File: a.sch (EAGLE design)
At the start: 22 parts, among them SW1 TS6601-9,5, SW2 TS6601-9,5, U1 ESP32-WROVER-IE, X1 PLS-09, X2 PLS-07, X3 PLS2-6, X4 PLD-06

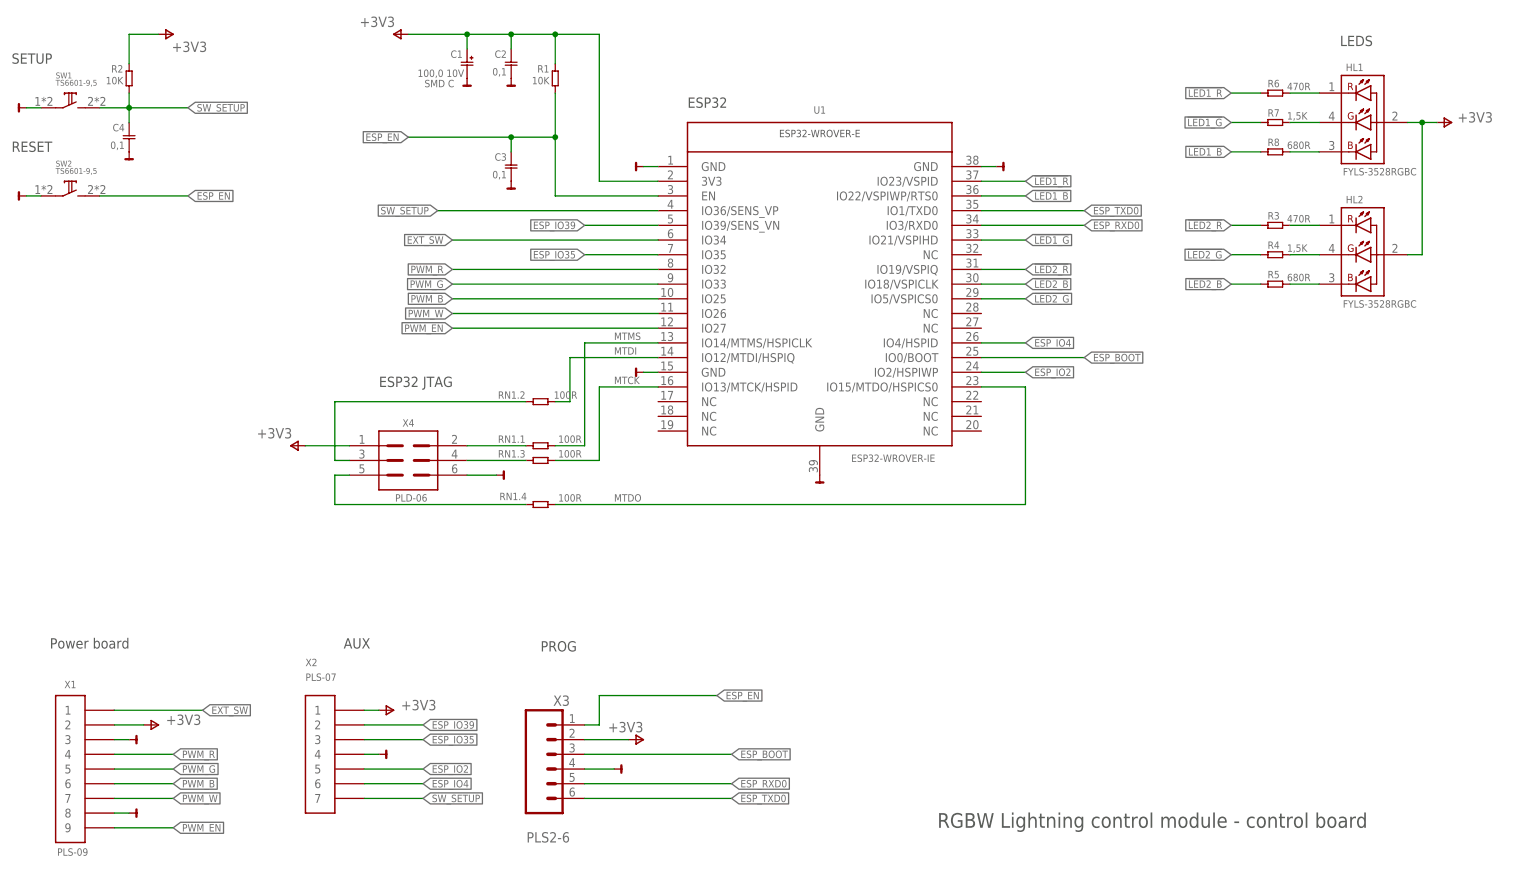
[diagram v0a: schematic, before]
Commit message: more import
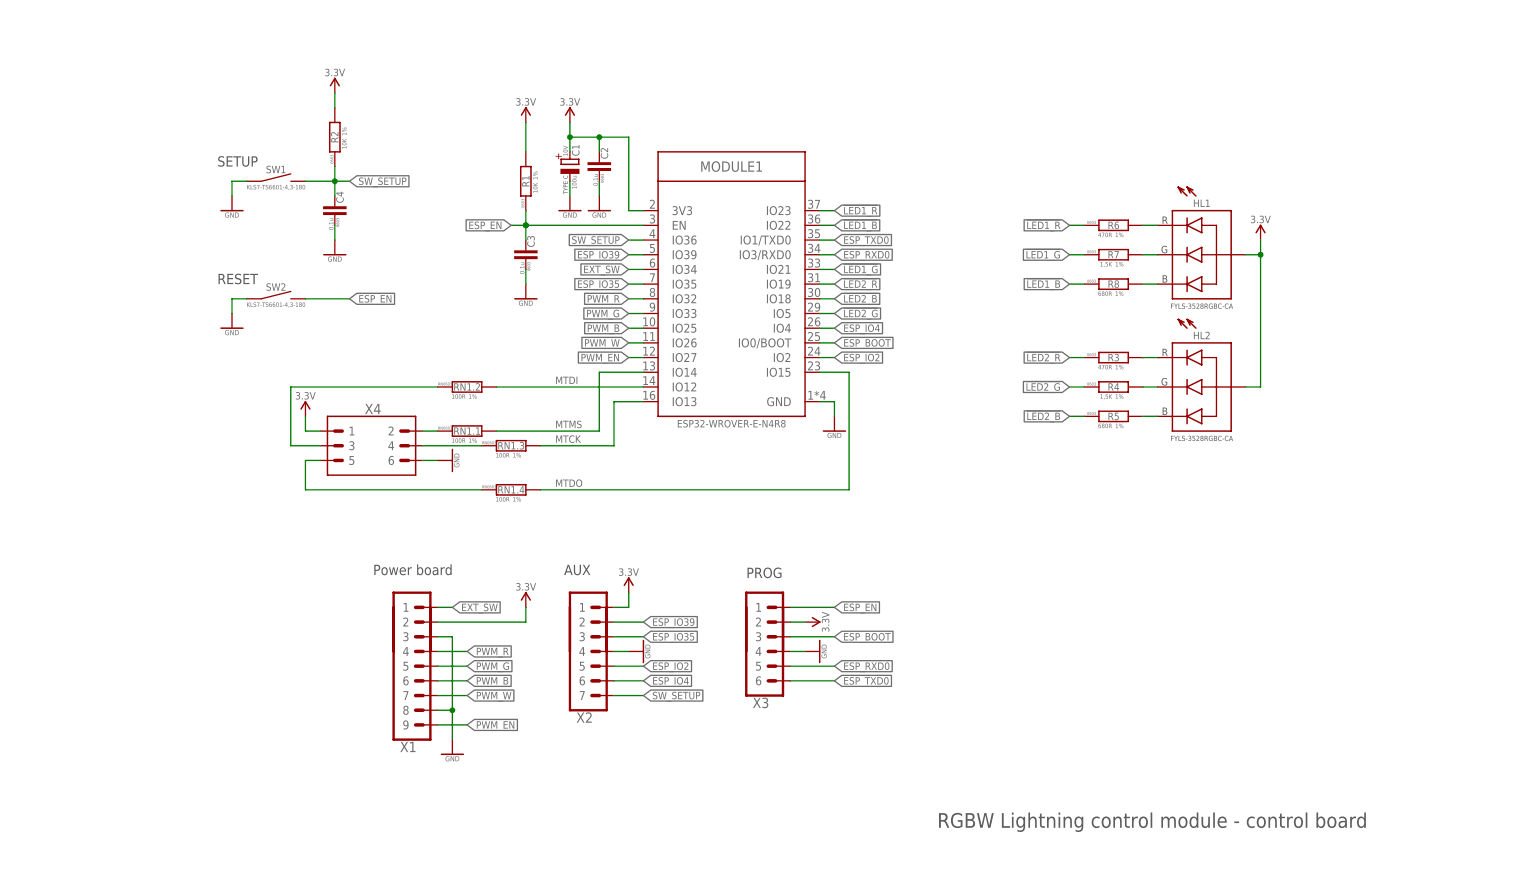
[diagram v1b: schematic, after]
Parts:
- removed U1: ESP32-WROVER-IE, pds019_lit:ESP32-WROVER-(I)E
- added MODULE1: ESP32-WROVER-(I)E, ali_modules:ESP32-WROVER-(I)E
- C1: value 100,0 10V -> 100u; device pds019_lit:CTANT_C -> rc:CPOL-TANT-TYPE-C; PKG SMD C -> (none); VOLTAGE (none) -> 10V
- C2, C3, C4: value 0,1 -> 0.1u; device pds019_lit:C0603 -> rc:C-0603; PKG 0603 -> (none); TOL -20/+80% -> (none); TYPE Y5V -> (none)
- HL1, HL2: value FYLS-3528RGBC -> LED_RGB-3528; device pds019_lit:FYLS-3528RGBC -> rc:LED_RGB-3528
- R1, R2, R3, R4, R5, R6, R7, R8: device pds019_lit:R0603 -> rc:R-1%-0603; PKG 0603 -> (none); TOL 5% -> (none)
- RN1: device pds019_lit:RN4X1_EXP-YC164 -> rc:RN-1%-0603
- SW1, SW2: device pds019_lit:SW_BUTTON -> mechanical:TACT_SWITCH-6X6-PTH
- X1: value PLS-09 -> PINHEAD_1X09-2.54-TH-MALE; device pds019_lit:PLS-09 -> pinhead:PINHEAD_1X09-2.54-TH-MALE
- X2: value PLS-07 -> PINHEAD_1X07-2.54; device pds019_lit:PLS-07 -> pinhead:PINHEAD_1X07-2.54
- X3: value PLS2-6 -> PINHEAD_1X06-2-MALE; device pds019_lit:PLS2-6 -> pinhead:PINHEAD_1X06-2-MALE
- X4: value PLD-06 -> PINHEAD_2X03-PTH-2.54; device pds019:PLD-06 -> pinhead:PINHEAD_2X03-PTH-2.54
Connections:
- removed net +3V3: C1.+, C2.2, HL1.A, HL2.A, R1.P$2, R2.P$2, U1.3V3, X1.2, X2.1, X3.2, X4.1
- new net VDD_3V3: C1.+, C2.2, HL1.A, HL2.A, MODULE1.3V3, R1.2, R2.2, X1.2, X2.1, X3.2, X4.1
- net !LED1_B: now also MODULE1.IO22, R8.1; no longer R8.P$1, U1.IO22/VSPIWP/RTS0
- net !LED1_G: now also MODULE1.IO21, R7.1; no longer R7.P$1, U1.IO21/VSPIHD
- net !LED1_R: now also MODULE1.IO23, R6.1; no longer R6.P$1, U1.IO23/VSPID
- net !LED2_B: now also MODULE1.IO18, R5.1; no longer R5.P$1, U1.IO18/VSPICLK
- net !LED2_G: now also MODULE1.IO5, R4.1; no longer R4.P$1, U1.IO5/VSPICS0
- net !LED2_R: now also MODULE1.IO19, R3.1; no longer R3.P$1, U1.IO19/VSPIQ
- net ESP_BOOT: now also MODULE1.IO0/BOOT; no longer U1.IO0/BOOT
- net ESP_EN: now also MODULE1.EN, R1.1; no longer R1.P$1, U1.EN
- net ESP_IO2: now also MODULE1.IO2; no longer U1.IO2/HSPIWP
- net ESP_IO35: now also MODULE1.IO35; no longer U1.IO35
- net ESP_IO39: now also MODULE1.IO39; no longer U1.IO39/SENS_VN
- net ESP_IO4: now also MODULE1.IO4; no longer U1.IO4/HSPID
- net ESP_RXD0: now also MODULE1.IO3/RXD0; no longer U1.IO3/RXD0
- net ESP_TXD0: now also MODULE1.IO1/TXD0; no longer U1.IO1/TXD0
- net EXT_SW: now also MODULE1.IO34; no longer U1.IO34
- net GND: now also MODULE1.GND; no longer U1.GND@1, U1.GND@15, U1.GND@38, U1.GND@39
- net MTCK: now also MODULE1.IO13, RN1.3.2; no longer RN1.3.P$2, U1.IO13/MTCK/HSPID
- net MTDI: now also MODULE1.IO12, RN1.2.2; no longer RN1.2.P$2, U1.IO12/MTDI/HSPIQ
- net MTDI_J: now also RN1.2.1; no longer RN1.2.P$1
- net MTDO: now also MODULE1.IO15, RN1.4.2; no longer RN1.4.P$2, U1.IO15/MTDO/HSPICS0
- net MTMS: now also MODULE1.IO14, RN1.1.2; no longer RN1.1.P$2, U1.IO14/MTMS/HSPICLK
- net N$1: now also R3.2; no longer R3.P$2
- net N$2: now also R7.2; no longer R7.P$2
- net N$3: now also R6.2; no longer R6.P$2
- net N$4: now also R8.2; no longer R8.P$2
- net N$5: now also R4.2; no longer R4.P$2
- net N$6: now also RN1.1.1; no longer RN1.1.P$1
- net N$7: now also RN1.3.1; no longer RN1.3.P$1
- net N$8: now also RN1.4.1; no longer RN1.4.P$1
- net N$9: now also R5.2; no longer R5.P$2
- net PWM_B: now also MODULE1.IO25; no longer U1.IO25
- net PWM_EN: now also MODULE1.IO27; no longer U1.IO27
- net PWM_G: now also MODULE1.IO33; no longer U1.IO33
- net PWM_R: now also MODULE1.IO32; no longer U1.IO32
- net PWM_W: now also MODULE1.IO26; no longer U1.IO26
- net SW_SETUP: now also MODULE1.IO36, R2.1; no longer R2.P$1, U1.IO36/SENS_VP
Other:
- note removed: "ESP32"
- note removed: "ESP32 JTAG"
- note removed: "LEDS"
